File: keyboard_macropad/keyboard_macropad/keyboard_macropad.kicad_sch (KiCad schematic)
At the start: 42 parts, among them J1 Conn_01x04_Pin, J2 Conn_01x04_Pin, J3 Conn_01x04_Pin, J4 Conn_01x04_Pin, SW1 SW_Push, SW10 SW_Push, SW11 SW_Push, SW12 SW_Push, SW13 SW_Push, SW14 SW_Push, SW15 SW_Push, SW16 SW_Push, SW2 SW_Push, SW3 SW_Push, SW4 SW_Push, SW5 SW_Push, SW6 SW_Push, SW7 SW_Push, SW8 SW_Push, SW9 SW_Push, U1 XIAO-RP2040-DIP

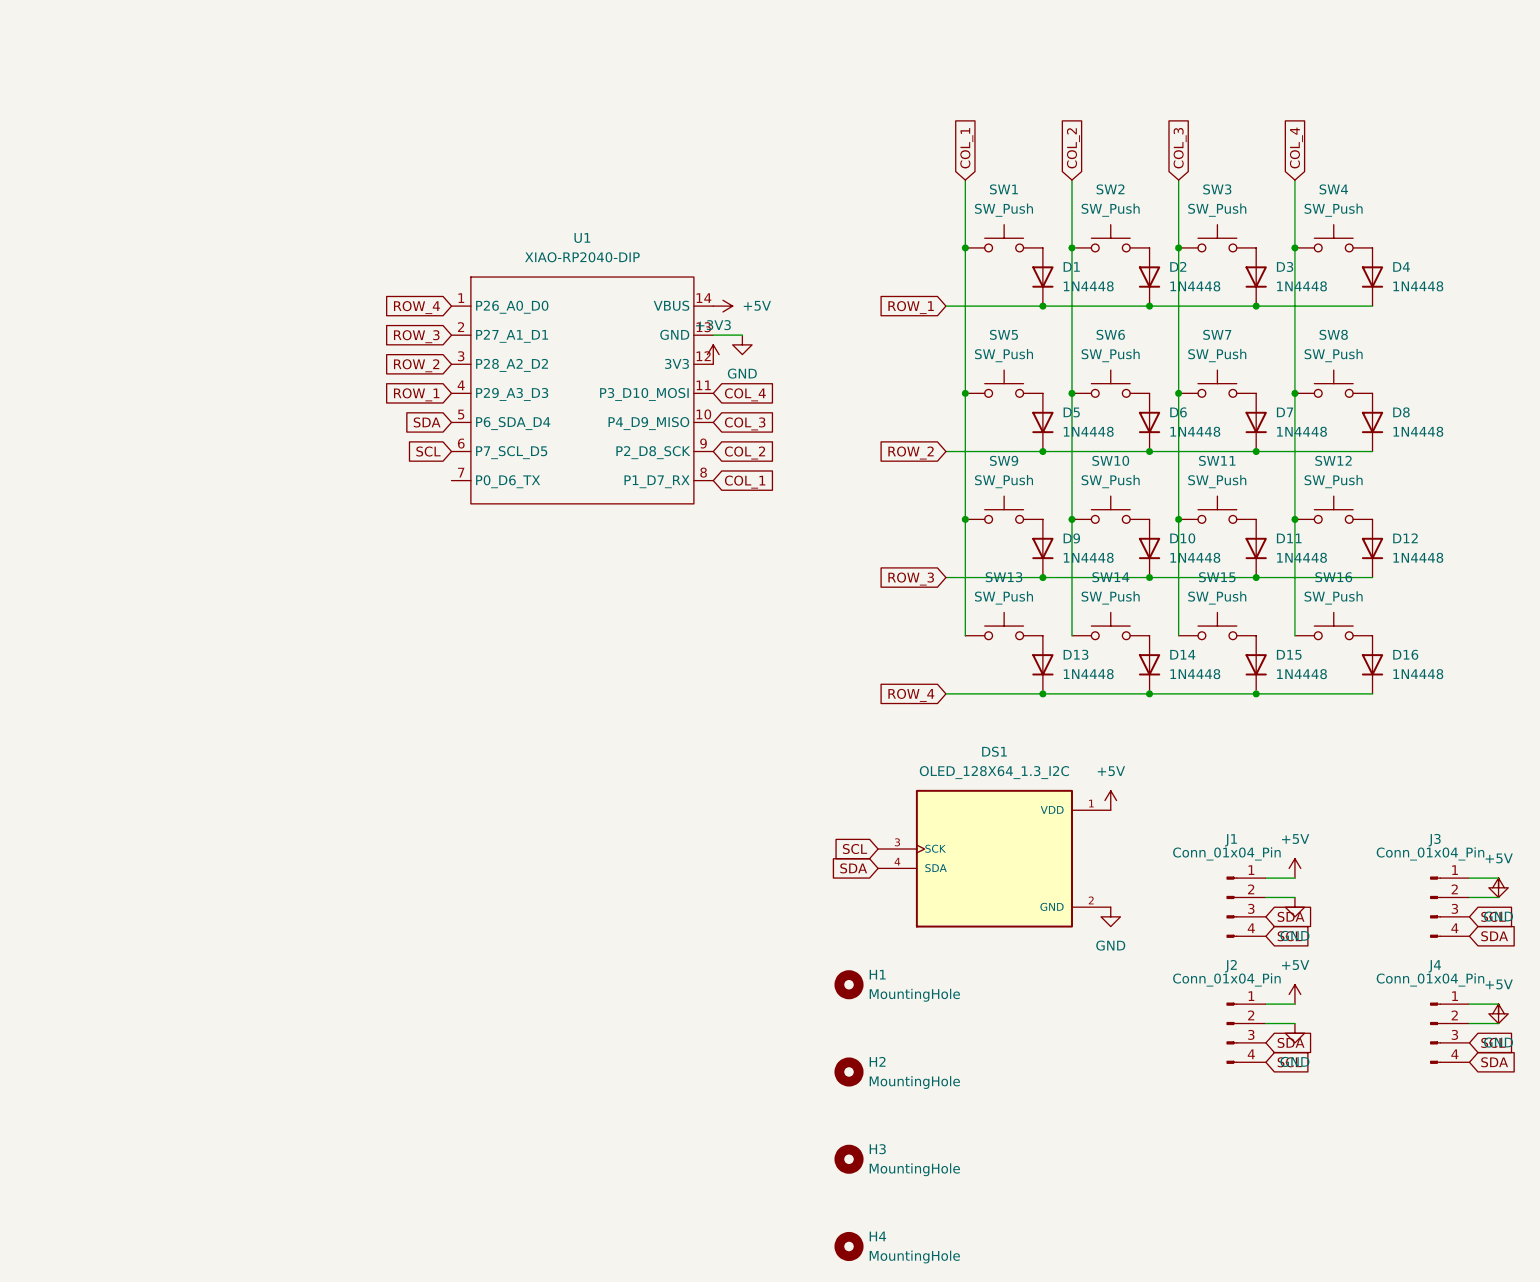
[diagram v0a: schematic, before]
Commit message: updates
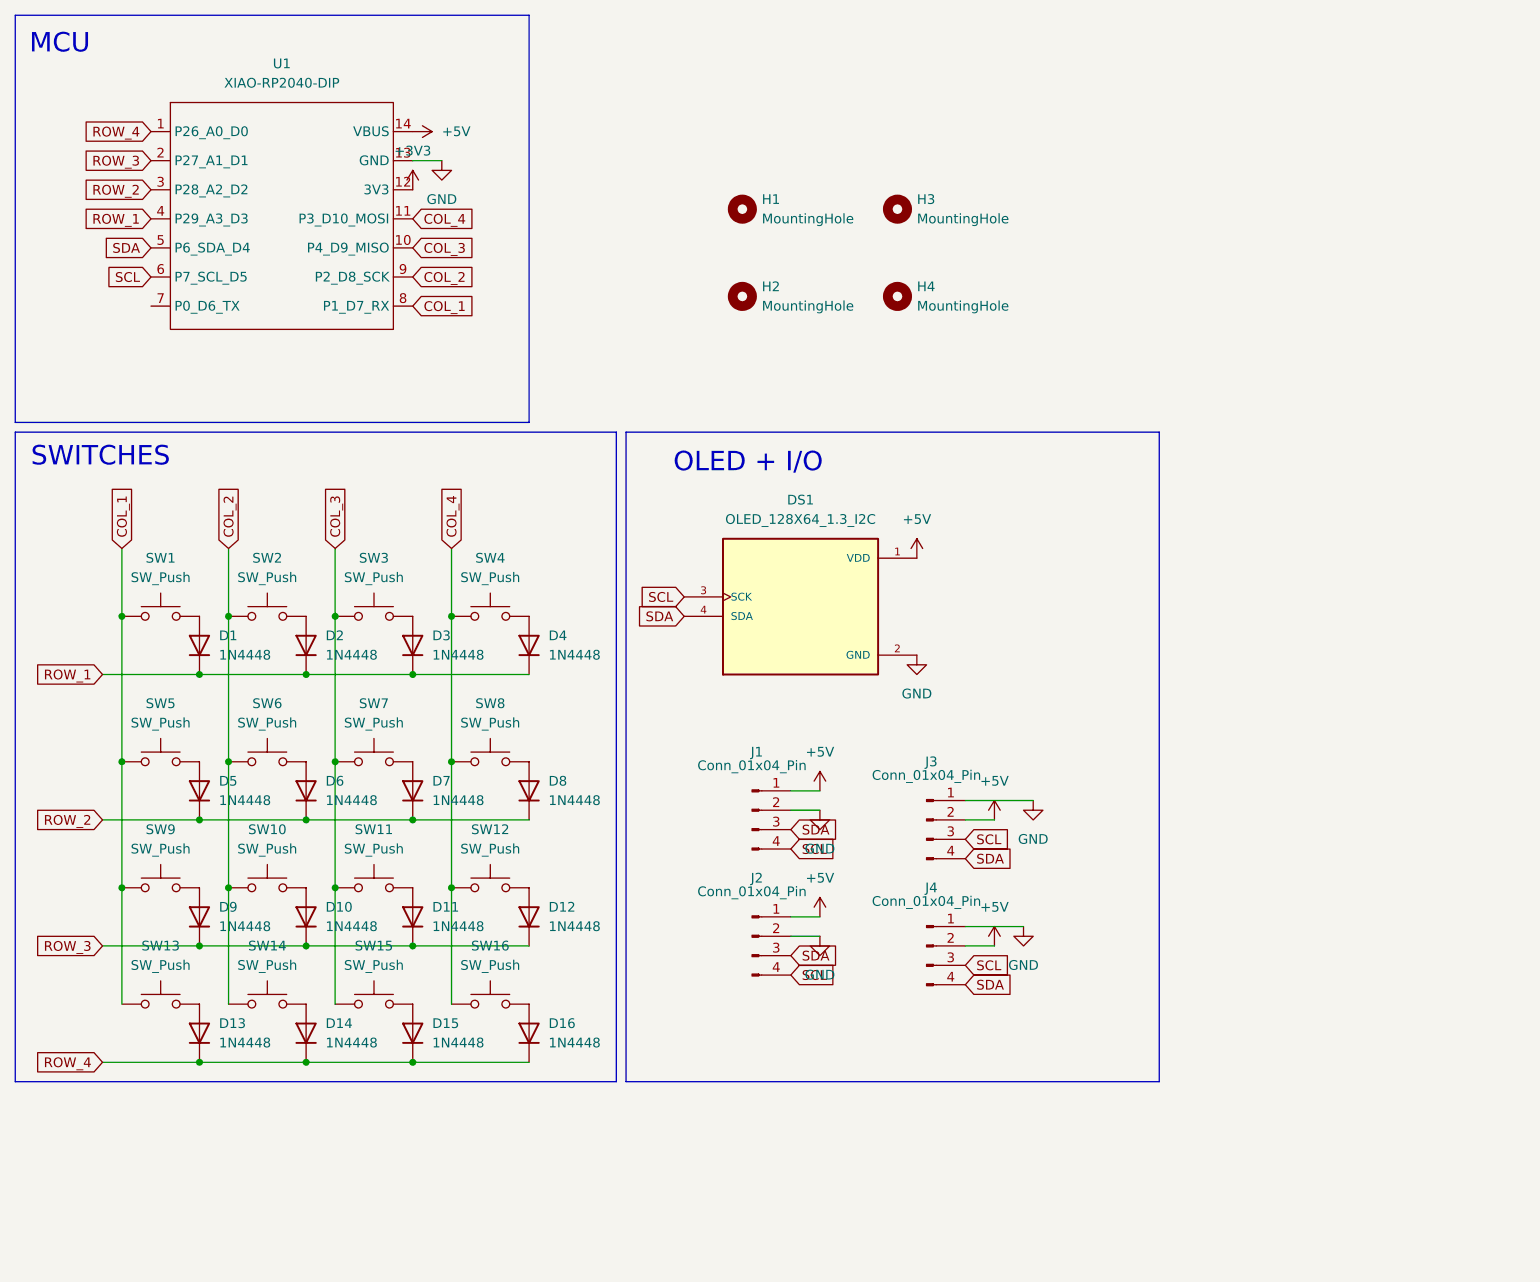
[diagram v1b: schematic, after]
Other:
- note added: "MCU"
- note added: "OLED + I/O"
- note added: "SWITCHES"
- moved on the sheet: D1, D10, D11, D12, D13, D14, D15, D16, D2, D3, D4, D5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
